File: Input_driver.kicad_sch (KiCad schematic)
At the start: 12 parts, among them J1001 5.08mm 2P Screw Plug-in Termi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, J1002 5.08mm 2P Screw Plug-in Termi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, U1001 PC817, U1002 PC817

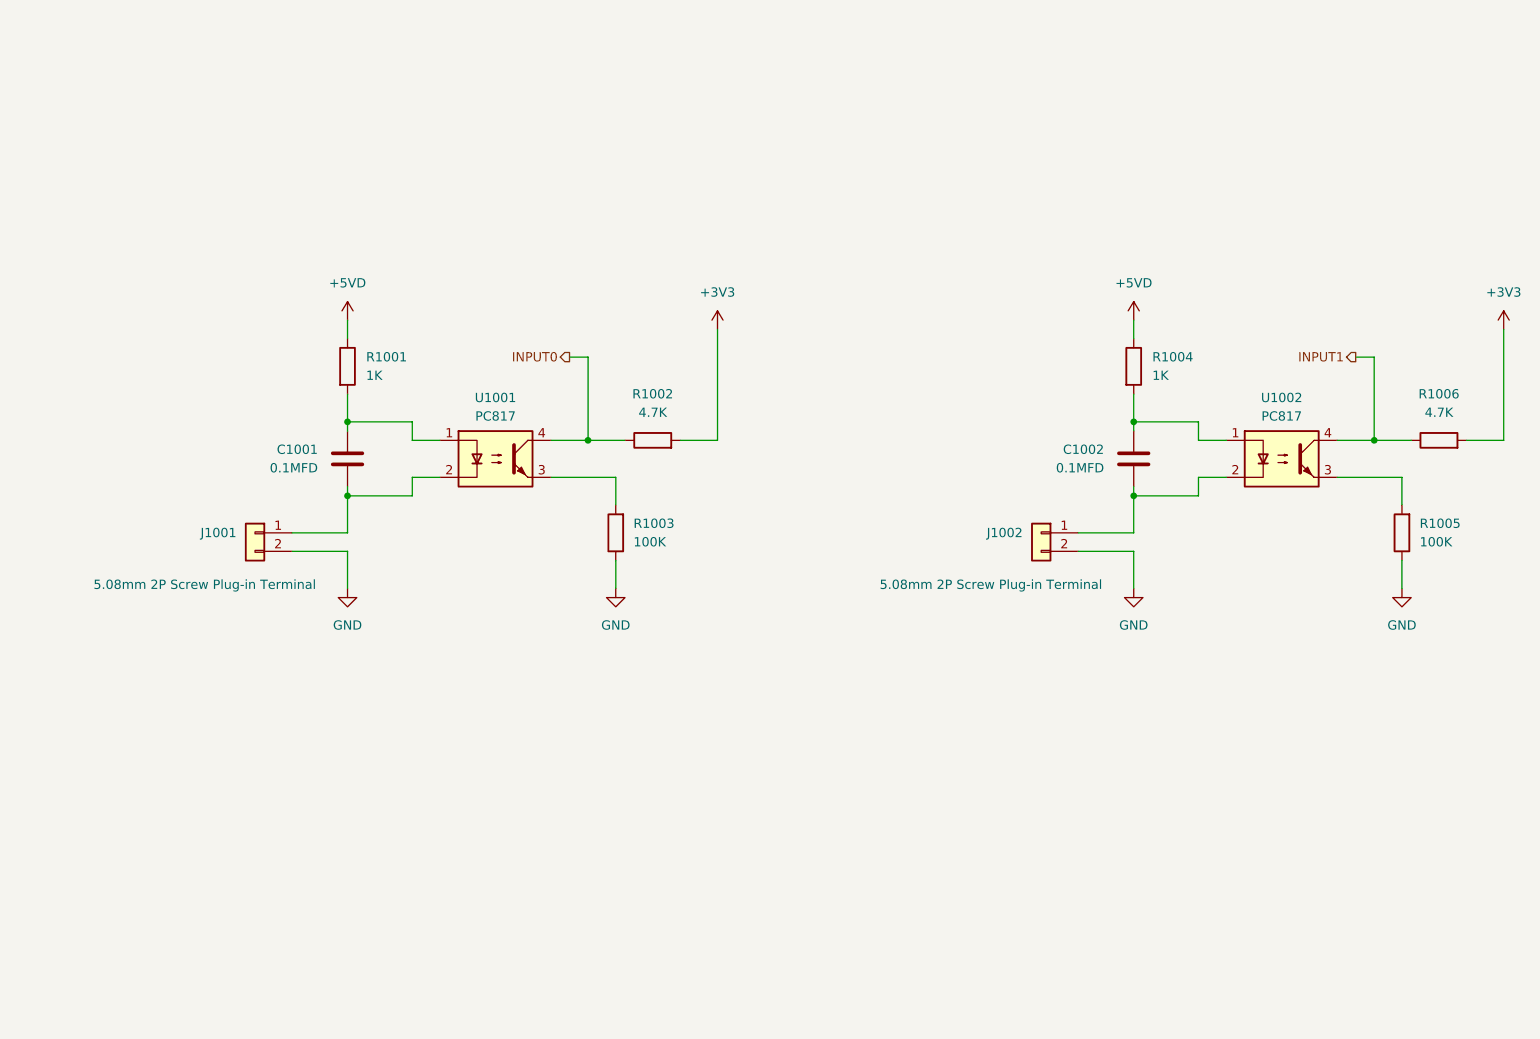
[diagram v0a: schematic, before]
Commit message: "V1.0 final design"
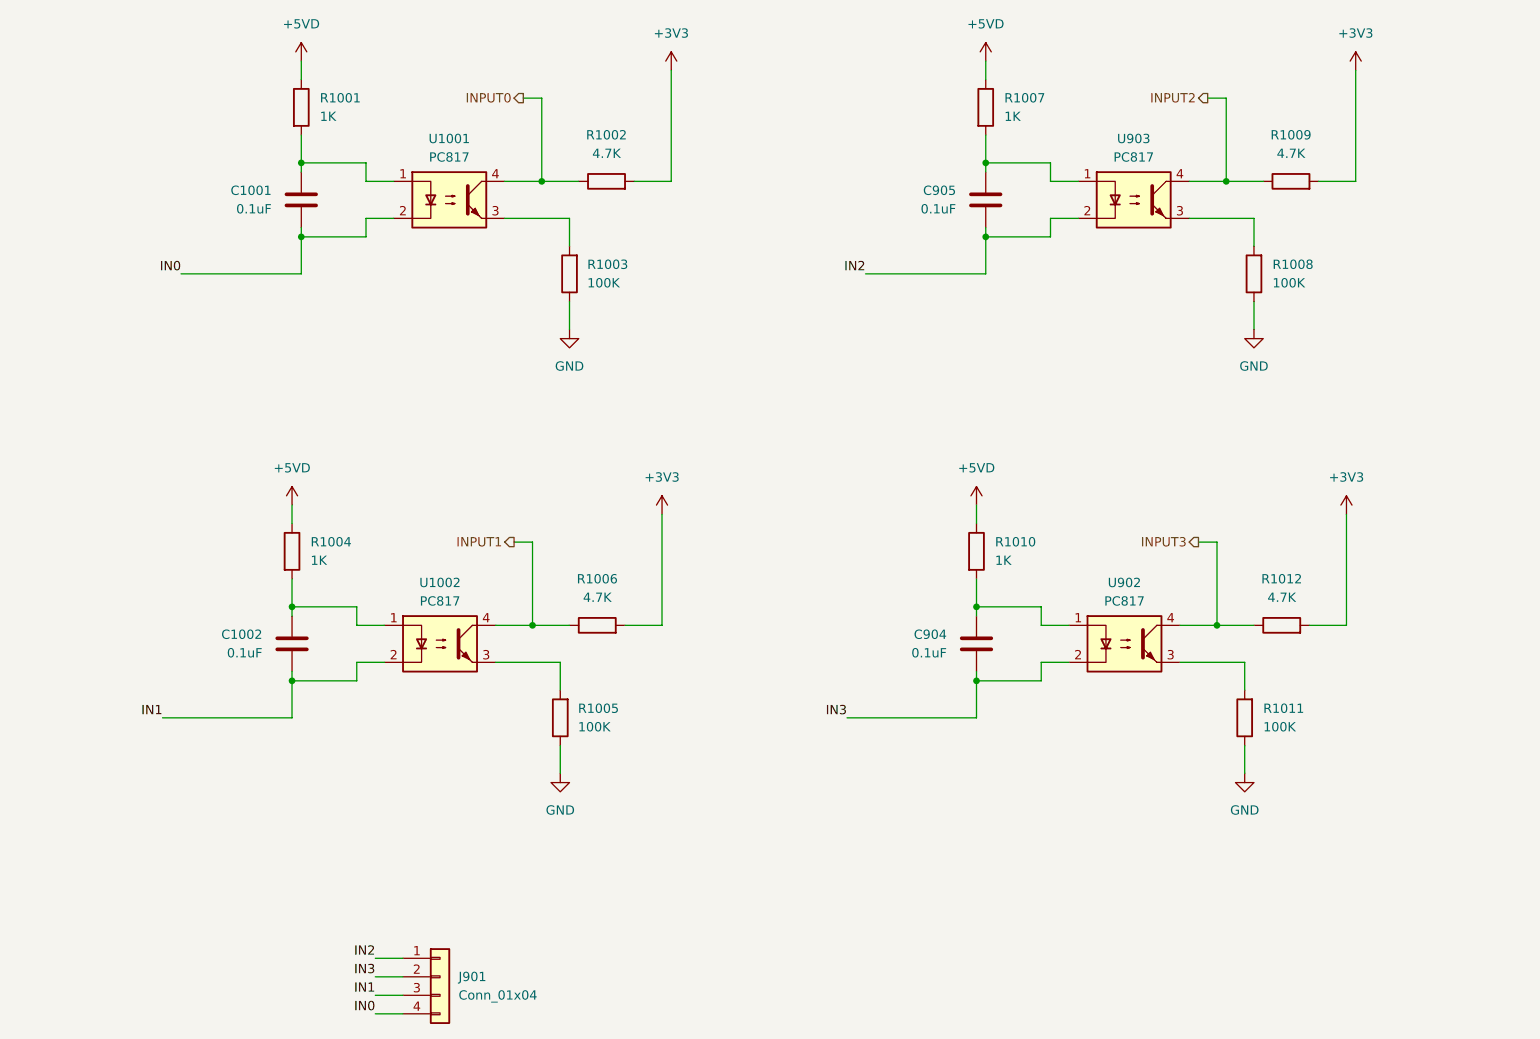
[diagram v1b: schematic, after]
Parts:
- removed J1001, J1002: 5.08mm 2P Screw Plug-in Terminal, Connector_Phoenix_MSTB:PhoenixContact_MSTBA_2,5_2-G-5,08_1x02_P5.08mm_Horizontal, symbol Connector_Generic:Conn_01x02
- added C904, C905: 0.1uF, Capacitor_SMD:C_0402_1005Metric_Pad0.74x0.62mm_HandSolder, symbol Device:C
- added J901: Conn_01x04, Connector_Phoenix_MC_HighVoltage:PhoenixContact_MCV_1,5_4-G-5.08_1x04_P5.08mm_Vertical, symbol Connector_Generic:Conn_01x04
- added R1007, R1010: 1K, Resistor_SMD:R_0603_1608Metric_Pad0.98x0.95mm_HandSolder, symbol Device:R
- added R1008, R1011: 100K, Resistor_SMD:R_0402_1005Metric_Pad0.72x0.64mm_HandSolder, symbol Device:R
- added R1009, R1012: 4.7K, Resistor_SMD:R_0402_1005Metric_Pad0.72x0.64mm_HandSolder, symbol Device:R
- added U902, U903: PC817, Package_DIP:DIP-4_W7.62mm, symbol Isolator:PC817
- C1001, C1002: value 0.1MFD -> 0.1uF
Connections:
- net +3V3: now also R1009.2, R1012.2
- net +5VD: now also R1007.1, R1010.1
- net GND: now also R1008.1, R1011.1
- net IN1: now reaches C1002.2, U1002.2
- net IN1: now also J901.3 (Pin_3)
- net IN0: now reaches C1001.2, U1001.2
- net IN0: now also J901.4 (Pin_4)
- new net: C905.1, R1007.2, U903.1
- new net: R1008.2, U903.3
- new net: C904.1, R1010.2, U902.1
- new net: R1011.2, U902.3
- new net IN2: C905.2, J901.1 (Pin_1), U903.2
- new net IN3: C904.2, J901.2 (Pin_2), U902.2
- new net INPUT2: R1009.1, U903.4
- new net INPUT3: R1012.1, U902.4
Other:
- moved on the sheet: C1001, C1002, R1001, R1002, R1003, R1004, R1005, R1006, U1001, U1002
